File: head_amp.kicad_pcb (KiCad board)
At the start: 4 copper layers, 50 x 50 mm, 53 parts, among them J1 Conn_01x15, J2 Conn_01x15, J3 Conn_01x05, J4 Conn_01x03, J5 Left_Speaker, J6 Left_Speaker, J7 Left_Speaker, J8 Left_Speaker, M1 Fan, Q1 AO3401A, Q2 AO3400A, U2 Headphone Jack, U3 WM8988LGECN/V, U4 WM8988LGECN/V

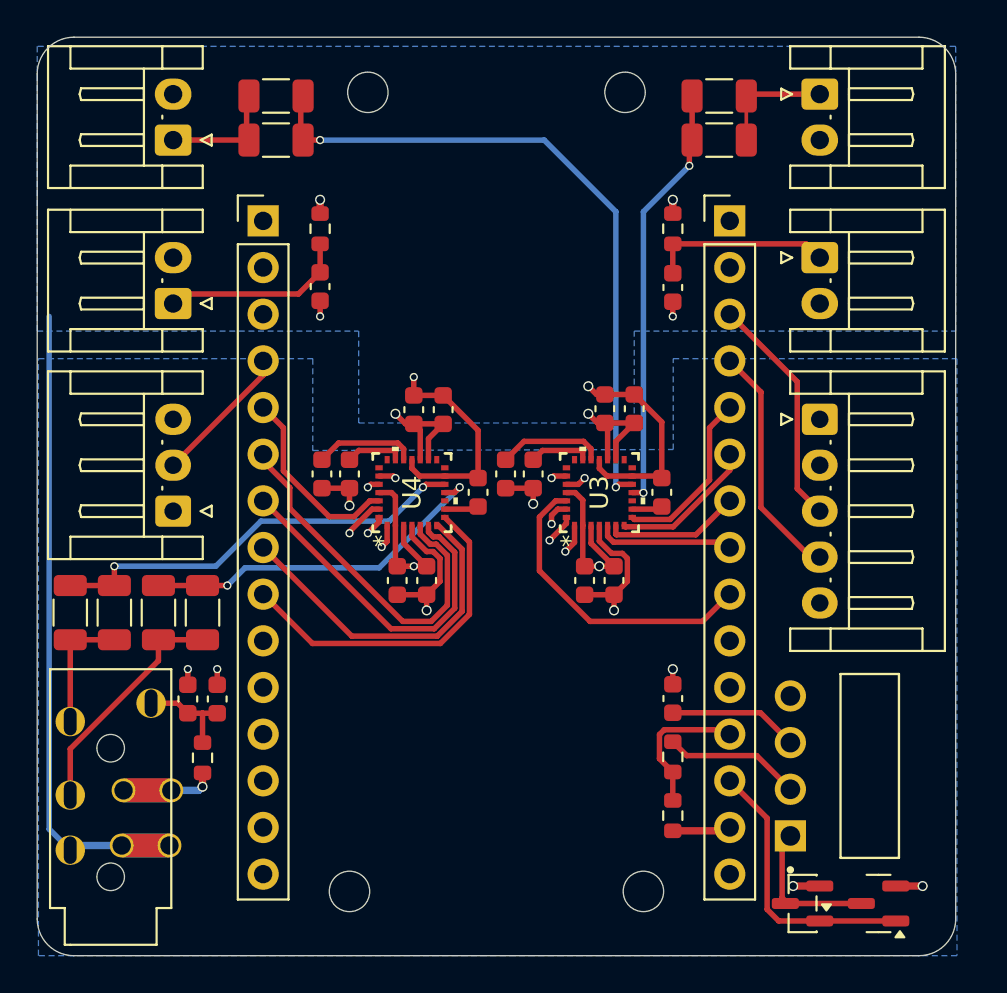
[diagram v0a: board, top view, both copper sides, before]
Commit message: feat: overhaul
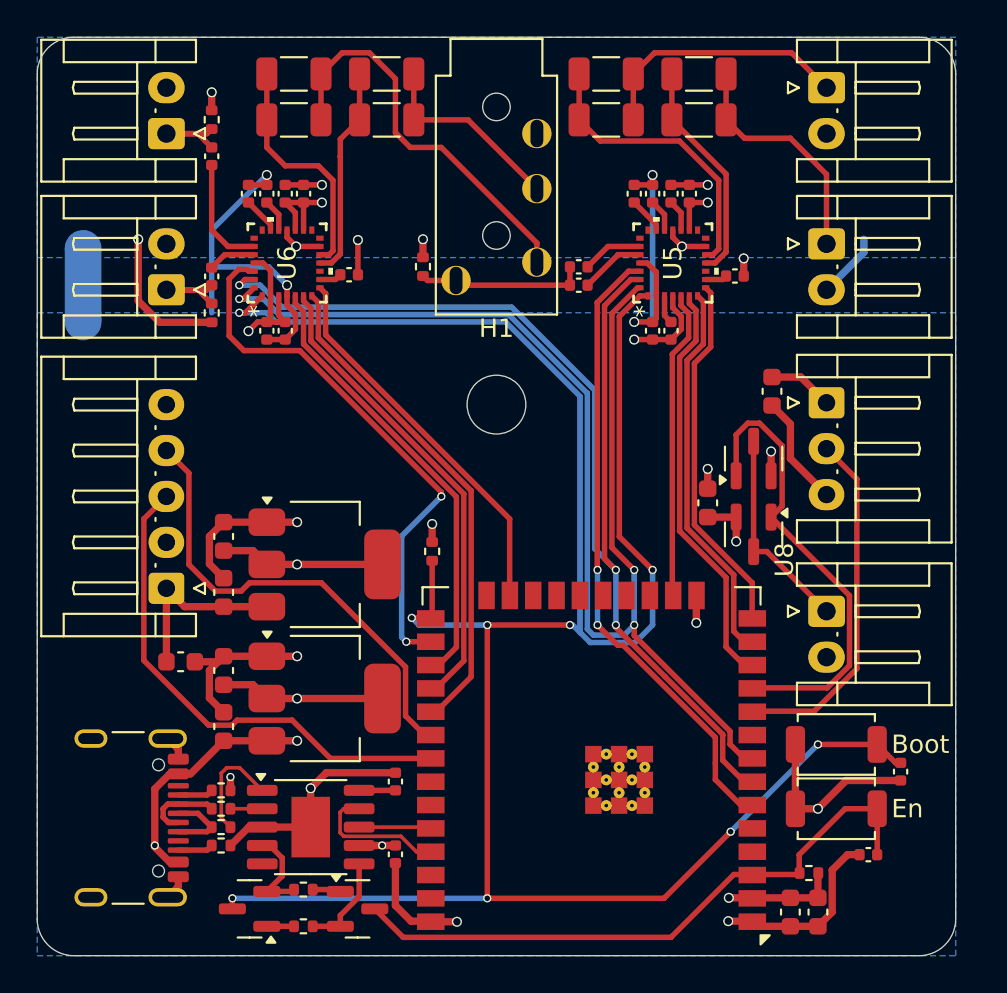
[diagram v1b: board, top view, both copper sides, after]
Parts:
- removed C11: 4.7u, Capacitor_SMD:C_0603_1608Metric
- removed H2, H3, H4: MountingHole, MountingHole:MountingHole_2.2mm_M2
- removed M1: Fan, A2543WR-4P:MOLEX_22053041
- removed NT1: NetTie_2, NetTie:NetTie-2_THT_Pad1.0mm
- removed U3: WM8988LGECN/V, footprints:QFN28_4X4_CIR
- added C2: 100n, Capacitor_SMD:C_0603_1608Metric, F.Cu at (130.8, 110.0)
- added C3: 22u, Capacitor_SMD:C_0603_1608Metric, F.Cu at (133.2, 110.5)
- added C30: 100u, Capacitor_SMD:C_1206_3216Metric, F.Cu at (137.0, 80.5)
- added C31: 100u, Capacitor_SMD:C_1206_3216Metric, F.Cu at (137.0, 78.0)
- added C32: 4.7u, Capacitor_SMD:C_0402_1005Metric, F.Cu at (134.5, 84.5)
- added C33: 4.7u, Capacitor_SMD:C_0402_1005Metric, F.Cu at (135.5, 84.5)
- added C34: 1u, Capacitor_SMD:C_0402_1005Metric, F.Cu at (132.5, 89.0)
- added C35: 4.7u, Capacitor_SMD:C_0402_1005Metric, F.Cu at (137.5, 84.5)
- added C36: 4.7u, Capacitor_SMD:C_0402_1005Metric, F.Cu at (136.5, 84.5)
- added C37: 1u, Capacitor_SMD:C_0402_1005Metric, F.Cu at (132.5, 82.5)
- added C38: 100n, Capacitor_SMD:C_0603_1608Metric, F.Cu at (159.5, 101.3)
- added C39: 10u, Capacitor_SMD:C_0603_1608Metric, F.Cu at (133.2, 106.2)
- added C40: 22u, Capacitor_SMD:C_0603_1608Metric, F.Cu at (133.2, 103.2)
- added Q3: AO3401A, Package_TO_SOT_SMD:SOT-23, F.Cu at (162.0, 103.1)
- added Q4: AO3400A, Package_TO_SOT_SMD:SOT-23, F.Cu at (162.0, 98.9)
- added R10: 10k, Resistor_SMD:R_0402_1005Metric, F.Cu at (132.5, 80.5)
- added R13: 10k, Resistor_SMD:R_0402_1005Metric, F.Cu at (165.0, 121.5)
- added R14: 10k, Resistor_SMD:R_0402_1005Metric, F.Cu at (144.5, 104.0)
- added R6: 10k, Resistor_SMD:R_0402_1005Metric, F.Cu at (137.5, 124.4)
- added R8: 10k, Resistor_SMD:R_0402_1005Metric, F.Cu at (132.5, 91.0)
- added R9: 10k, Resistor_SMD:R_0402_1005Metric, F.Cu at (144.0, 88.5)
- added SW1: SW_Push, Button_Switch_SMD:SW_SPST_TS-1088-xR020, F.Cu at (166.5, 114.5)
- added SW2: SW_Push, Button_Switch_SMD:SW_SPST_TS-1088-xR020, F.Cu at (166.5, 118.0)
- added U1: AMS1117-3.3, Package_TO_SOT_SMD:SOT-223-3_TabPin2, F.Cu at (138.7, 112.0)
- added U5: WM8988LGECN/V, footprints:QFN28_4X4_CIR, F.Cu at (157.6, 88.3)
- added U6: WM8988LGECN/V, footprints:QFN28_4X4_CIR, F.Cu at (136.6, 88.3)
- added U7: AMS1117-3.3, Package_TO_SOT_SMD:SOT-223-3_TabPin2, F.Cu at (138.7, 104.7)
- added U8: ESP32-WROOM-32E, RF_Module:ESP32-WROOM-32E, F.Cu at (153.2, 118.9)
- C1: value 100n -> 10u
- C10: value 100u -> 1u; footprint Capacitor_SMD:C_1206_3216Metric -> Capacitor_SMD:C_0603_1608Metric
- C12, C15, C25, C28, C8: value 4.7u -> 100n; footprint Capacitor_SMD:C_0603_1608Metric -> Capacitor_SMD:C_0402_1005Metric
- C13, C26: value 1u -> 100u; footprint Capacitor_SMD:C_0603_1608Metric -> Capacitor_SMD:C_1206_3216Metric
- C14, C27: value 4.7u -> 100u; footprint Capacitor_SMD:C_0603_1608Metric -> Capacitor_SMD:C_1206_3216Metric
- C16, C29: value 1u -> 4.7u; footprint Capacitor_SMD:C_0603_1608Metric -> Capacitor_SMD:C_0402_1005Metric
- C17: value 100n -> 100u; footprint Capacitor_SMD:C_0603_1608Metric -> Capacitor_SMD:C_1206_3216Metric
- C19, C22, C23: value 100u -> 4.7u; footprint Capacitor_SMD:C_1206_3216Metric -> Capacitor_SMD:C_0402_1005Metric
- C20: value 100n -> 4.7u; footprint Capacitor_SMD:C_0603_1608Metric -> Capacitor_SMD:C_0402_1005Metric
- C21, C24: value 4.7u -> 1u; footprint Capacitor_SMD:C_0603_1608Metric -> Capacitor_SMD:C_0402_1005Metric
- C5, C6: value 100u -> 100n; footprint Capacitor_SMD:C_1206_3216Metric -> Capacitor_SMD:C_0402_1005Metric
- C7: footprint Capacitor_SMD:C_0603_1608Metric -> Capacitor_SMD:C_0402_1005Metric
- C9: value 100u -> 100n; footprint Capacitor_SMD:C_1206_3216Metric -> Capacitor_SMD:C_0603_1608Metric
- H1: footprint MountingHole:MountingHole_2.2mm_M2 -> MountingHole:MountingHole_3.2mm_M3
- J1: value Conn_01x15 -> USB Port; footprint Connector_PinHeader_2.54mm:PinHeader_1x15_P2.54mm_Vertical -> Connector_USB:USB_C_Receptacle_GCT_USB4105-xx-A_16P_TopMnt_Horizontal
- J2: value Conn_01x15 -> I2C; footprint Connector_PinHeader_2.54mm:PinHeader_1x15_P2.54mm_Vertical -> Connector_JST:JST_EH_S5B-EH_1x05_P2.50mm_Horizontal
- J3: value Conn_01x05 -> LED; footprint Connector_JST:JST_EH_S5B-EH_1x05_P2.50mm_Horizontal -> Connector_JST:JST_EH_S3B-EH_1x03_P2.50mm_Horizontal
- J4: value Conn_01x03 -> Left_Mic; footprint Connector_JST:JST_EH_S3B-EH_1x03_P2.50mm_Horizontal -> Connector_JST:JST_EH_S2B-EH_1x02_P2.50mm_Horizontal
- J6: value Left_Speaker -> Right_Mic
- J7: value Left_Speaker -> Right_Speaker
- J8: value Left_Speaker -> Fan
- NT2: footprint NetTie:NetTie-2_THT_Pad1.0mm -> NetTie:NetTie-2_SMD_Pad2.0mm; moved to B.Cu
- Q1: value AO3401A -> MMBT3904
- Q2: value AO3400A -> MMBT3904
- R1: value 50k -> 22; footprint Resistor_SMD:R_0603_1608Metric -> Resistor_SMD:R_0402_1005Metric
- R2: value 27k -> 22; footprint Resistor_SMD:R_0603_1608Metric -> Resistor_SMD:R_0402_1005Metric
- R3, R4: value 10k -> 5.1k; footprint Resistor_SMD:R_0603_1608Metric -> Resistor_SMD:R_0402_1005Metric
- R5: footprint Resistor_SMD:R_0603_1608Metric -> Resistor_SMD:R_0402_1005Metric
- U2: value Headphone Jack -> CH340K; footprint PJ-320A:PJ-320A -> Package_SO:SSOP-10-1EP_3.9x4.9mm_P1mm_EP2.1x3.3mm
- U4: value WM8988LGECN/V -> Headphone Jack; footprint footprints:QFN28_4X4_CIR -> PJ-320A:PJ-320A
- moved C9 52.5 mm to (164.0, 123.6), turned to 90 degrees
- moved C10 51.3 mm to (165.5, 123.6), turned to -90 degrees
- moved C13 43.0 mm to (159.0, 78.0), turned to 180 degrees
- moved C5 42.7 mm to (142.5, 120.5), turned to 90 degrees
- moved R4 41.6 mm to (133.0, 120.0), turned to 0 degrees
- moved C6 41.3 mm to (142.5, 116.5), turned to 90 degrees
- moved C22 40.7 mm to (158.5, 84.5), turned to -90 degrees
- moved C23 37.9 mm to (157.5, 84.5), turned to -90 degrees
- moved C16 37.6 mm to (161.0, 89.0), turned to 0 degrees
- moved C18 36.6 mm to (154.0, 78.0), turned to 180 degrees
- moved J2 36.6 mm to (130.0, 106.0), turned to 90 degrees
- moved J5 35.7 mm to (166.0, 78.8), turned to -90 degrees
- moved C19 34.5 mm to (155.5, 84.5), turned to -90 degrees
- moved J1 33.5 mm to (127.0, 118.5), turned to -90 degrees
- moved R3 31.0 mm to (133.0, 117.0), turned to 0 degrees
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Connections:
- C1 pad 1: +5V -> GND
- C1 pad 2: GND -> +5V
- C10 pad 1: /Speaker_Left -> +3V3D
- C10 pad 2: Net-(U3-LOUT1) -> GND
- C12 pad 2: Net-(U3-VREF) -> +3V3D
- C13 pad 1: /Headset_Mic -> /Speaker_Right
- C13 pad 2: Net-(U3-LINPUT1) -> Net-(U5-ROUT1)
- C14 pad 1: GNDA -> /Speaker_Right
- C14 pad 2: +3V3A -> Net-(U5-ROUT1)
- C15 pad 1: GNDA -> GND
- C15 pad 2: +3V3A -> +3V3D
- C16 pad 1: /Headset_Mic -> Net-(U5-HPCOM)
- C16 pad 2: Net-(U3-RINPUT1) -> GNDA
- C17 pad 1: GND -> /Speaker_Left
- C17 pad 2: +3V3D -> Net-(U5-LOUT1)
- C18 pad 1: /Headset_Right -> /Speaker_Left
- C18 pad 2: Net-(U4-ROUT1) -> Net-(U5-LOUT1)
- C19 pad 1: /Headset_Right -> GND
- C19 pad 2: Net-(U4-ROUT1) -> Net-(U5-VMID)
- C20 pad 2: +3V3D -> Net-(U5-VREF)
- C21 pad 1: Net-(U4-HPCOM) -> /Headset_Mic
- C21 pad 2: GNDA -> Net-(U5-LINPUT1)
- C22 pad 1: /Headset_Left -> GNDA
- C22 pad 2: Net-(U4-LOUT1) -> +3V3A
- C23 pad 1: /Headset_Left -> GNDA
- C23 pad 2: Net-(U4-LOUT1) -> +3V3A
- C24 pad 1: GND -> /Headset_Mic
- C24 pad 2: Net-(U4-VMID) -> Net-(U5-RINPUT1)
- C25 pad 2: Net-(U4-VREF) -> +3V3D
- C26 pad 1: /Mic_Left -> /Headset_Right
- C26 pad 2: Net-(U4-LINPUT1) -> Net-(U6-ROUT1)
- C27 pad 1: GNDA -> /Headset_Right
- C27 pad 2: +3V3A -> Net-(U6-ROUT1)
- C28 pad 1: GNDA -> GND
- C28 pad 2: +3V3A -> +3V3D
- C29 pad 1: /Mic_Right -> Net-(U6-HPCOM)
- C29 pad 2: Net-(U4-RINPUT1) -> GNDA
- C4 pad 1: GND -> +5V
- C4 pad 2: +3V3D -> GND
- C5 pad 1: /Speaker_Right -> GND
- C5 pad 2: Net-(U3-ROUT1) -> +3V3D
- C6 pad 1: /Speaker_Right -> Net-(U2-V3)
- C6 pad 2: Net-(U3-ROUT1) -> GND
- C7 pad 2: +3V3D -> /GPIO0
- C8 pad 1: Net-(U3-HPCOM) -> GND
- C8 pad 2: GNDA -> /MCU_EN
- C9 pad 1: /Speaker_Left -> GND
- C9 pad 2: Net-(U3-LOUT1) -> +3V3D
- J2 pad 1: unconnected-(J2-Pin_1-Pad1) -> +5V
- J2 pad 2: unconnected-(J2-Pin_2-Pad2) -> +3V3D
- J2 pad 5: /Int->Ext_Out -> GND
- J3 pad 2: +3V3D -> /LED_Data
- J3 pad 3: /Out_DAT -> GND
- J4 pad 1: +5V -> /Mic_Left
- J4 pad 2: /LED_Data -> GNDA
- J6 pad 1: /Mic_Left -> /Mic_Right
- J8 pad 1: /Mic_Right -> Net-(J8-Pin_1)
- J8 pad 2: GNDA -> GND
- Q1 pad 1: /FAN_PWM -> Net-(Q1-B)
- Q1 pad 2: +5V -> /RTS
- Q1 pad 3: Net-(M1-PWM) -> /MCU_EN
- Q2 pad 1: /FAN_PWM -> Net-(Q2-B)
- Q2 pad 2: GND -> /DTR
- Q2 pad 3: Net-(M1-PWM) -> /GPIO0
- R1 pad 1: GND -> Net-(J1-D--PadA7)
- R1 pad 2: /FAN_RPM -> /USB_D-
- R2 pad 1: /FAN_RPM -> Net-(J1-D+-PadA6)
- R2 pad 2: Net-(M1-Tacho) -> /USB_D+
- R3 pad 1: /Mic_Left -> Net-(J1-CC1)
- R3 pad 2: +3V3A -> GND
- R4 pad 1: /Mic_Right -> Net-(J1-CC2)
- R4 pad 2: +3V3A -> GND
- R5 pad 1: +3V3A -> /DTR
- R5 pad 2: /Headset_Mic -> Net-(Q1-B)
- U2 pad 1: /Headset_Mic -> /USB_D+
- U2 pad 2: /Headset_Left -> /USB_D-
- U2 pad 3: /Headset_Right -> GND
- U2 pad 4: GNDA -> /DTR
- U4 pad 1: /Master_Audio_Clk -> /Headset_Mic
- U4 pad 2: +3V3D -> /Headset_Left
- U4 pad 3: +3V3D -> /Headset_Right
- U4 pad 4: GND -> GNDA
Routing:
- net /GPIO0: track 0.00 -> 128.6 mm, vias 0 -> 9
- net GND: track 25.2 -> 102.6 mm, vias 6 -> 14
- net /SPI_CLK: track 23.6 -> 67.6 mm, vias 2 -> 3
- net /MOSI: track 22.7 -> 64.9 mm, vias 2 -> 3
- net GNDA: track 56.6 -> 15.3 mm, vias 2 -> 6
- net Net-(U3-LOUT1): track 37.2 -> 0.00 mm, vias 2 -> 0
- net /MCU_EN: track 0.00 -> 34.0 mm
- net /Ext->Int_Select: track 0.00 -> 30.7 mm, vias 0 -> 2
- net Net-(U3-LINPUT1): track 26.3 -> 0.00 mm, vias 2 -> 0
- net /Master_Audio_Clk: track 25.9 -> 0.00 mm, vias 2 -> 0
- net Net-(U3-RINPUT1): track 25.8 -> 0.00 mm, vias 2 -> 0
- net /Fan_PWM: track 0.00 -> 25.2 mm
- net Net-(U3-ROUT1): track 23.3 -> 0.00 mm, vias 2 -> 0
- net Net-(U4-LOUT1): track 23.3 -> 0.00 mm, vias 2 -> 0
- net +5V: track 8.54 -> 29.9 mm, vias 1 -> 3
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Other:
- board text added: "Boot"
- board text added: "En"
- board text added: "Fan"
- board text added: "I2C"
- board text added: "LED"
- board text added: "Left"
- board text added: "Microphone"
- board text added: "Right"
- board text added: "Speaker"
